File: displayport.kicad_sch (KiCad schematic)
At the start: 1 part, among them J2 DP_Source

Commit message: Add files via upload
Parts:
- J2: footprint (none) -> DPF20102741TR:AMPHENOL_DPF20102741TR
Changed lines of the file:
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@@
 			)
 		)
-		(property "Footprint" ""
+		(property "Footprint" "DPF20102741TR:AMPHENOL_DPF20102741TR"
 			(at 120.65 97.79 0)
 			(hide yes)

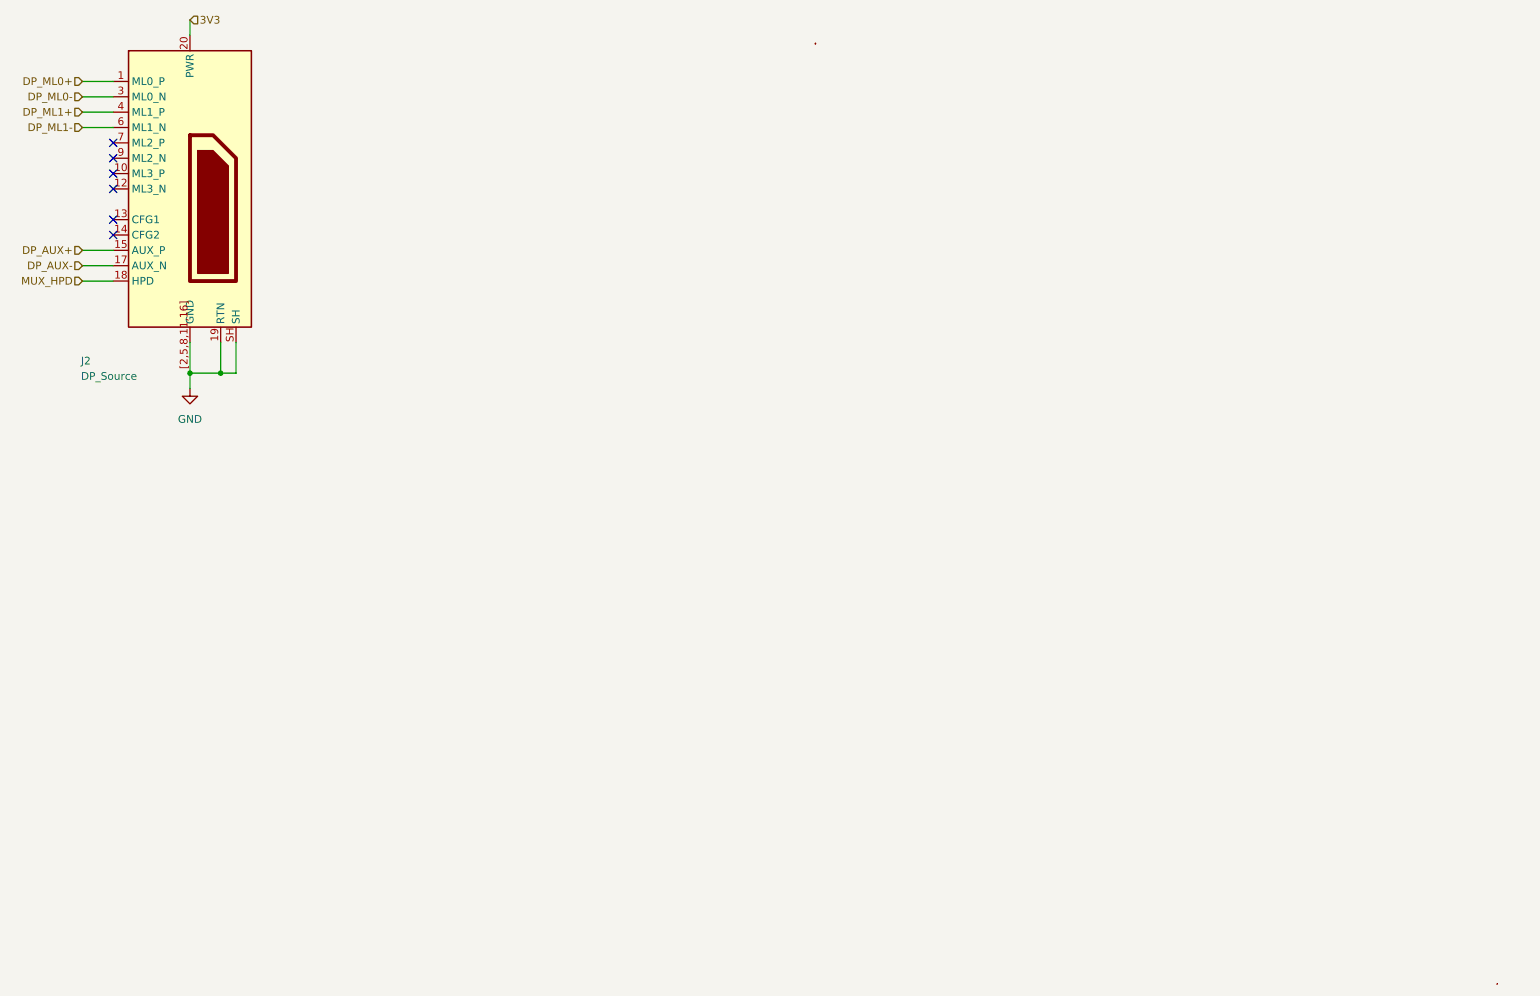
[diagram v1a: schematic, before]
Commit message: Add files via upload
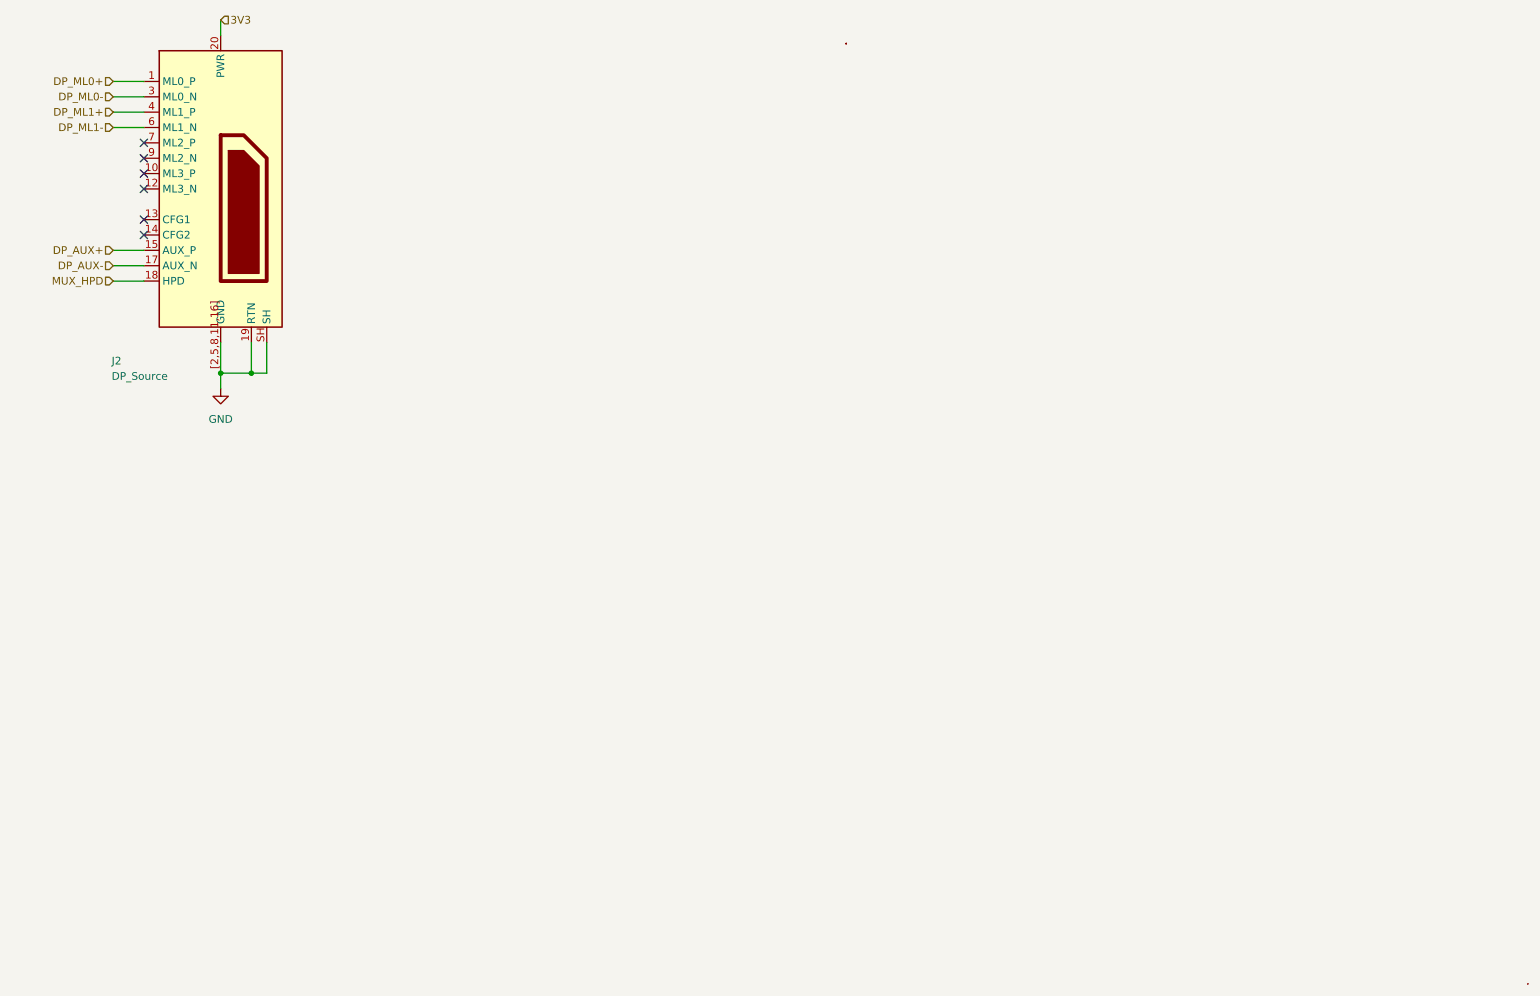
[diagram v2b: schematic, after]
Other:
- moved on the sheet: J2
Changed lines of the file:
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@@
+	)
+	(junction
+		(at 130.81 128.27)
+		(diameter 0)
+		(color 0 0 0 0)
 	)
 	(junction
@@
 		(color 0 0 0 0)
 	)
-	(junction
-		(at 120.65 128.27)
-		(diameter 0)
-		(color 0 0 0 0)
-	)
-	(no_connect
-		(at 107.95 95.25)
-	)
-	(no_connect
-		(at 107.95 102.87)
-	)
-	(no_connect
-		(at 107.95 90.17)
-	)
-	(no_connect
-		(at 107.95 92.71)
-	)
-	(no_connect
-		(at 107.95 97.79)
-	)
-	(no_connect
-		(at 107.95 105.41)
-	)
-	(wire
-		(pts
-			(xy 125.73 128.27) (xy 128.27 128.27)
-		)
-		(stroke
-			(width 0)
-			(type default)
-		)
-	)
-	(wire
-		(pts
-			(xy 120.65 130.81) (xy 120.65 128.27)
-		)
-		(stroke
-			(width 0)
-			(type default)
-		)
-	)
-	(wire
-		(pts
-			(xy 128.27 123.19) (xy 128.27 128.27)
-		)
-		(stroke
-			(width 0)
-			(type default)
-		)
-	)
-	(wire
-		(pts
-			(xy 120.65 128.27) (xy 125.73 128.27)
+	(no_connect
+		(at 113.03 95.25)
+	)
+	(no_connect
+		(at 113.03 102.87)
+	)
+	(no_connect
+		(at 113.03 90.17)
+	)
+	(no_connect
+		(at 113.03 92.71)
+	)
+	(no_connect
+		(at 113.03 97.79)
+	)
+	(no_connect
+		(at 113.03 105.41)
+	)
+	(wire
+		(pts
+			(xy 130.81 128.27) (xy 133.35 128.27)
+		)
+		(stroke
+			(width 0)
+			(type default)
+		)
+	)
+	(wire
+		(pts
+			(xy 125.73 130.81) (xy 125.73 128.27)
+		)
+		(stroke
+			(width 0)
+			(type default)
+		)
+	)
+	(wire
+		(pts
+			(xy 133.35 123.19) (xy 133.35 128.27)
+		)
+		(stroke
+			(width 0)
+			(type default)
+		)
+	)
+	(wire
+		(pts
+			(xy 125.73 128.27) (xy 130.81 128.27)
+		)
+		(stroke
+			(width 0)
+			(type default)
+		)
+	)
+	(wire
+		(pts
+			(xy 130.81 123.19) (xy 130.81 128.27)
+		)
+		(stroke
+			(width 0)
+			(type default)
+		)
+	)
+	(wire
+		(pts
+			(xy 113.03 107.95) (xy 107.95 107.95)
+		)
+		(stroke
+			(width 0)
+			(type default)
+		)
+	)
+	(wire
+		(pts
+			(xy 113.03 82.55) (xy 107.95 82.55)
+		)
+		(stroke
+			(width 0)
+			(type default)
+		)
+	)
+	(wire
+		(pts
+			(xy 113.03 110.49) (xy 107.95 110.49)
+		)
+		(stroke
+			(width 0)
+			(type default)
+		)
+	)
+	(wire
+		(pts
+			(xy 113.03 87.63) (xy 107.95 87.63)
+		)
+		(stroke
+			(width 0)
+			(type default)
+		)
+	)
+	(wire
+		(pts
+			(xy 113.03 85.09) (xy 107.95 85.09)
+		)
+		(stroke
+			(width 0)
+			(type default)
+		)
+	)
+	(wire
+		(pts
+			(xy 125.73 69.85) (xy 125.73 72.39)
+		)
+		(stroke
+			(width 0)
+			(type default)
+		)
+	)
+	(wire
+		(pts
+			(xy 113.03 113.03) (xy 107.95 113.03)
 		)
 		(stroke
@@
 	(wire
 		(pts
-			(xy 107.95 107.95) (xy 102.87 107.95)
-		)
-		(stroke
-			(width 0)
-			(type default)
-		)
-	)
-	(wire
-		(pts
-			(xy 107.95 82.55) (xy 102.87 82.55)
-		)
-		(stroke
-			(width 0)
-			(type default)
-		)
-	)
-	(wire
-		(pts
-			(xy 107.95 110.49) (xy 102.87 110.49)
-		)
-		(stroke
-			(width 0)
-			(type default)
-		)
-	)
-	(wire
-		(pts
-			(xy 107.95 87.63) (xy 102.87 87.63)
-		)
-		(stroke
-			(width 0)
-			(type default)
-		)
-	)
-	(wire
-		(pts
-			(xy 107.95 85.09) (xy 102.87 85.09)
-		)
-		(stroke
-			(width 0)
-			(type default)
-		)
-	)
-	(wire
-		(pts
-			(xy 120.65 69.85) (xy 120.65 72.39)
-		)
-		(stroke
-			(width 0)
-			(type default)
-		)
-	)
-	(wire
-		(pts
-			(xy 107.95 113.03) (xy 102.87 113.03)
-		)
-		(stroke
-			(width 0)
-			(type default)
-		)
-	)
-	(wire
-		(pts
-			(xy 120.65 123.19) (xy 120.65 128.27)
-		)
-		(stroke
-			(width 0)
-			(type default)
-		)
-	)
-	(wire
-		(pts
-			(xy 107.95 80.01) (xy 102.87 80.01)
+			(xy 113.03 80.01) (xy 107.95 80.01)
 		)
 		(stroke
@@
 	(hierarchical_label "DP_AUX+"
 		(shape input)
-		(at 102.87 107.95 180)
+		(at 107.95 107.95 180)
+		(effects
+			(font
+				(size 1.27 1.27)
+			)
+			(justify right)
+		)
+	)
+	(hierarchical_label "DP_ML0+"
+		(shape input)
+		(at 107.95 80.01 180)
 		(effects
 			(font
@@
 	(hierarchical_label "DP_ML0-"
 		(shape input)
-		(at 102.87 82.55 180)
-		(effects
-			(font
-				(size 1.27 1.27)
-			)
-			(justify right)
-		)
-	)
-	(hierarchical_label "DP_ML0+"
-		(shape input)
-		(at 102.87 80.01 180)
+		(at 107.95 82.55 180)
 		(effects
 			(font
@@
 	(hierarchical_label "MUX_HPD"
 		(shape input)
-		(at 102.87 113.03 180)
+		(at 107.95 113.03 180)
 		(effects
 			(font
@@
 	(hierarchical_label "DP_ML1+"
 		(shape input)
-		(at 102.87 85.09 180)
+		(at 107.95 85.09 180)
 		(effects
 			(font
@@
 	(hierarchical_label "3V3"
 		(shape input)
-		(at 120.65 69.85 0)
+		(at 125.73 69.85 0)
 		(effects
 			(font
@@
 	(hierarchical_label "DP_ML1-"
 		(shape input)
-		(at 102.87 87.63 180)
+		(at 107.95 87.63 180)
 		(effects
 			(font
@@
 	(hierarchical_label "DP_AUX-"
 		(shape input)
-		(at 102.87 110.49 180)
+		(at 107.95 110.49 180)
 		(effects
 			(font
@@
 	(symbol
 		(lib_id "power:GND")
-		(at 120.65 130.81 0)
+		(at 125.73 130.81 0)
 		(unit 1)
 		(body_style 1)
@@
 		(fields_autoplaced yes)
 		(property "Reference" "#PWR01"
-			(at 120.65 137.16 0)
+			(at 125.73 137.16 0)
 			(hide yes)
 			(show_name no)
@@
 		)
 		(property "Value" "GND"
-			(at 120.65 135.89 0)
+			(at 125.73 135.89 0)
 			(show_name no)
 			(do_not_autoplace no)
@@
 		)
 		(property "Footprint" ""
-			(at 120.65 130.81 0)
+			(at 125.73 130.81 0)
 			(hide yes)
 			(show_name no)
@@
 		)
 		(property "Datasheet" ""
-			(at 120.65 130.81 0)
+			(at 125.73 130.81 0)
 			(hide yes)
 			(show_name no)
@@
 		)
 		(property "Description" "Power symbol creates a global label with name \"GND\" , ground"
-			(at 120.65 130.81 0)
+			(at 125.73 130.81 0)
 			(hide yes)
 			(show_name no)
@@
 	(symbol
 		(lib_id "Connector:DP_Source")
-		(at 120.65 97.79 0)
+		(at 125.73 97.79 0)
 		(unit 1)
 		(body_style 1)
@@
 		(dnp no)
 		(property "Reference" "J2"
-			(at 102.616 126.238 0)
+			(at 107.696 126.238 0)
 			(show_name no)
 			(do_not_autoplace no)
@@
 		)
 		(property "Value" "DP_Source"
-			(at 102.616 128.778 0)
+			(at 107.696 128.778 0)
 			(show_name no)
 			(do_not_autoplace no)
@@
 		)
 		(property "Footprint" "DPF20102741TR:AMPHENOL_DPF20102741TR"
-			(at 120.65 97.79 0)
+			(at 125.73 97.79 0)
 			(hide yes)
 			(show_name no)
@@
 		)
 		(property "Datasheet" "https://en.wikipedia.org/wiki/DisplayPort"
-			(at 120.65 97.79 0)
+			(at 125.73 97.79 0)
 			(hide yes)
 			(show_name no)
@@
 		)
 		(property "Description" "Display port source connector"
-			(at 118.11 97.79 0)
-			(hide yes)
-			(show_name no)
+			(at 123.19 97.79 0)
+			(hide yes)
+			(show_name no)
